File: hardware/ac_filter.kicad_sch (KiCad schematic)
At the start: 3 parts

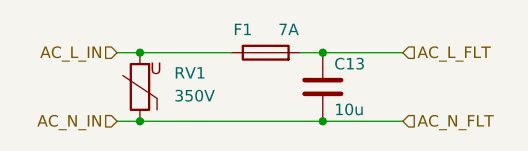
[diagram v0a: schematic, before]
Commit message: added some zones
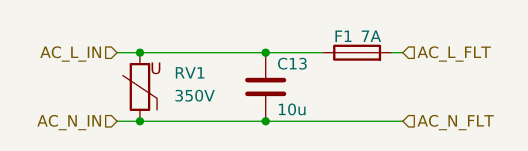
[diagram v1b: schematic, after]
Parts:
- F1: footprint Fuse:Fuse_Schurter_UMZ250 -> Fuse:Fuse_2512_6332Metric
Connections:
- net AC_L_FLT: no longer C13.1
- net AC_L_IN: now also C13.1
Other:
- moved on the sheet: C13, F1
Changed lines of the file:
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@@
-	)
-	(junction
-		(at 154.94 97.79)
-		(diameter 0)
-		(color 0 0 0 0)
 	)
 	(junction
@@
 	)
 	(junction
-		(at 154.94 90.17)
+		(at 148.59 90.17)
 		(diameter 0)
 		(color 0 0 0 0)
 	)
-	(wire
-		(pts
-			(xy 134.62 97.79) (xy 154.94 97.79)
-		)
-		(stroke
-			(width 0)
-			(type default)
-		)
-	)
-	(wire
-		(pts
-			(xy 154.94 90.17) (xy 163.83 90.17)
+	(junction
+		(at 148.59 97.79)
+		(diameter 0)
+		(color 0 0 0 0)
+	)
+	(wire
+		(pts
+			(xy 134.62 97.79) (xy 148.59 97.79)
+		)
+		(stroke
+			(width 0)
+			(type default)
+		)
+	)
+	(wire
+		(pts
+			(xy 148.59 97.79) (xy 163.83 97.79)
 		)
 		(stroke
@@
 	(wire
 		(pts
-			(xy 134.62 90.17) (xy 144.78 90.17)
-		)
-		(stroke
-			(width 0)
-			(type default)
-		)
-	)
-	(wire
-		(pts
-			(xy 152.4 90.17) (xy 154.94 90.17)
+			(xy 148.59 90.17) (xy 154.94 90.17)
+		)
+		(stroke
+			(width 0)
+			(type default)
+		)
+	)
+	(wire
+		(pts
+			(xy 134.62 90.17) (xy 148.59 90.17)
+		)
+		(stroke
+			(width 0)
+			(type default)
+		)
+	)
+	(wire
+		(pts
+			(xy 162.56 90.17) (xy 163.83 90.17)
 		)
 		(stroke
@@
 		(pts
 			(xy 132.08 90.17) (xy 134.62 90.17)
-		)
-		(stroke
-			(width 0)
-			(type default)
-		)
-	)
-	(wire
-		(pts
-			(xy 154.94 97.79) (xy 163.83 97.79)
 		)
 		(stroke
@@
 	(symbol
 		(lib_id "Device:C")
-		(at 154.94 93.98 0)
+		(at 148.59 93.98 0)
 		(unit 1)
 		(exclude_from_sim no)
@@
 		(dnp no)
 		(property "Reference" "C13"
-			(at 156.21 91.44 0)
+			(at 149.86 91.44 0)
 			(effects
 				(font
@@
 		)
 		(property "Value" "10u"
-			(at 156.21 96.52 0)
+			(at 149.86 96.52 0)
 			(effects
 				(font
@@
 		)
 		(property "Footprint" "Capacitor_THT:C_Disc_D16.0mm_W5.0mm_P10.00mm"
-			(at 155.9052 97.79 0)
+			(at 149.5552 97.79 0)
 			(effects
 				(font
@@
 		)
 		(property "Datasheet" "~"
-			(at 154.94 93.98 0)
+			(at 148.59 93.98 0)
 			(effects
 				(font
@@
 		)
 		(property "Description" ""
-			(at 154.94 93.98 0)
+			(at 148.59 93.98 0)
 			(effects
 				(font
@@
 	(symbol
 		(lib_id "Device:Fuse")
-		(at 148.59 90.17 90)
+		(at 158.75 90.17 90)
 		(unit 1)
 		(exclude_from_sim no)
@@
 		(dnp no)
 		(property "Reference" "F1"
-			(at 146.05 87.63 90)
+			(at 157.226 88.392 90)
 			(effects
 				(font
@@
 		)
 		(property "Value" "7A"
-			(at 151.13 87.63 90)
-			(effects
-				(font
-					(size 1.27 1.27)
-				)
-			)
-		)
-		(property "Footprint" "Fuse:Fuse_Schurter_UMZ250"
-			(at 148.59 91.948 90)
+			(at 160.274 88.392 90)
+			(effects
+				(font
+					(size 1.27 1.27)
+				)
+			)
+		)
+		(property "Footprint" "Fuse:Fuse_2512_6332Metric"
+			(at 158.75 91.948 90)
 			(effects
 				(font
@@
 		)
 		(property "Datasheet" "~"
-			(at 148.59 90.17 0)
+			(at 158.75 90.17 0)
 			(effects
 				(font
@@
 		)
 		(property "Description" ""
-			(at 148.59 90.17 0)
-			(effects
-				(font
+			(at 158.75 90.17 0)
+			(effects
+				(font
